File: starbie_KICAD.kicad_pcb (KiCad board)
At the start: 2 copper layers, 84.7 x 68 mm, 7 parts, among them J1 Conn_01x04_Pin, J2 Conn_01x08_Pin, SW1 SW_Push, SW2 SW_Push, U1 DHT11, U2 XIAO-ESP32-C3-SMD

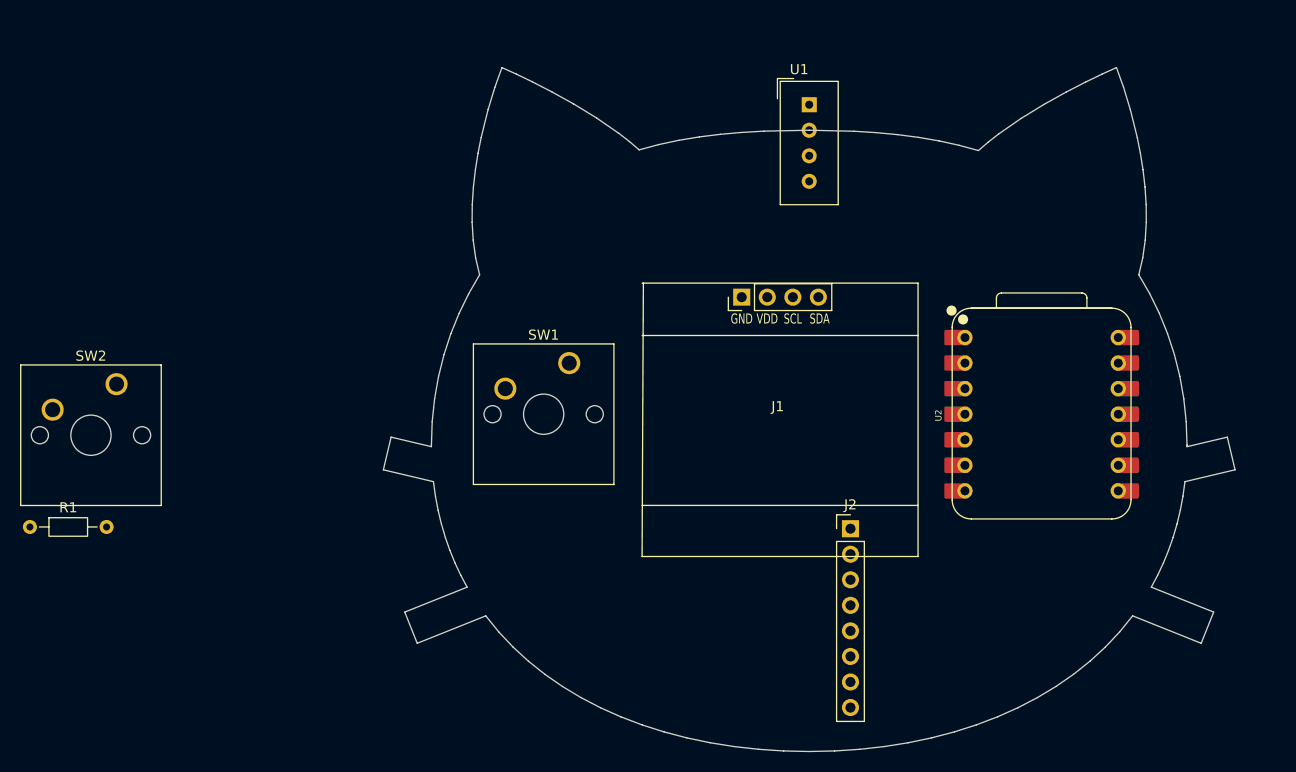
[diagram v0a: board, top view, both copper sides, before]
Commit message: Autosave
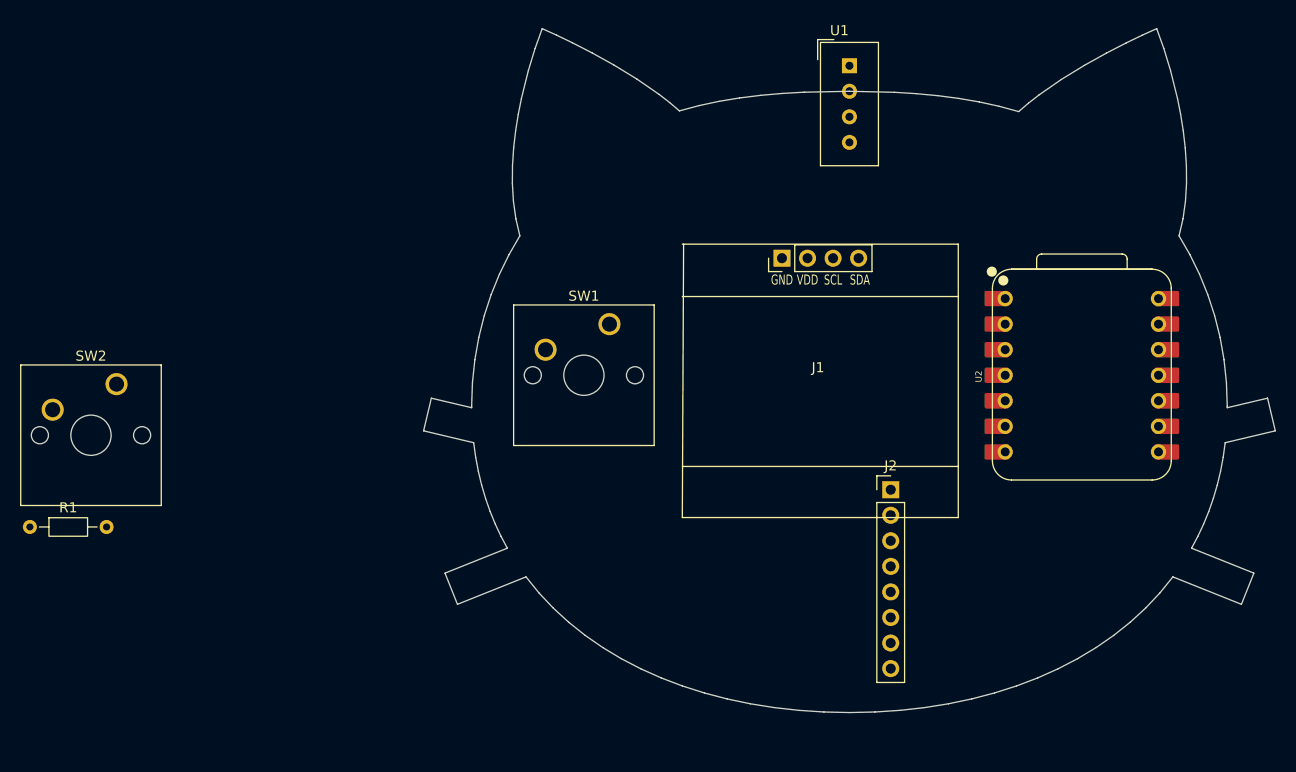
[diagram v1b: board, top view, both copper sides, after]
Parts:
- moved SW1 5.57 mm to (147.5, 74.5)
- moved U2 5.57 mm to (194.5, 79.6)
- moved U1 5.57 mm to (171.4, 48.9)
- moved J1 5.57 mm to (168.5, 68.0)
- moved J2 5.57 mm to (175.5, 91.0)
